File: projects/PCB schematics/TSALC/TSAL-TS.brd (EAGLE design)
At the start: 81.3 x 95.2 mm, 29 parts, among them J1 2P_1-770166-0, J2 2P_1-770166-0, J3 2P_1-770166-0, J4 2P_1-770166-0, X1 5566-2, X2 5566-2

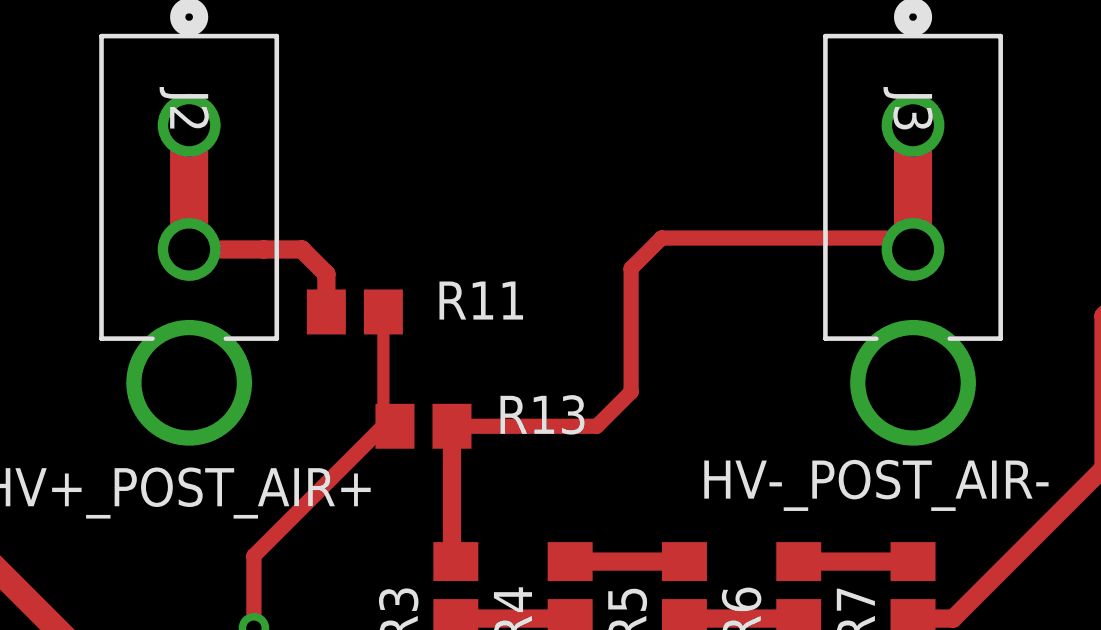
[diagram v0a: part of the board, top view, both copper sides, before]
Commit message: TSAL - Minor fixes.
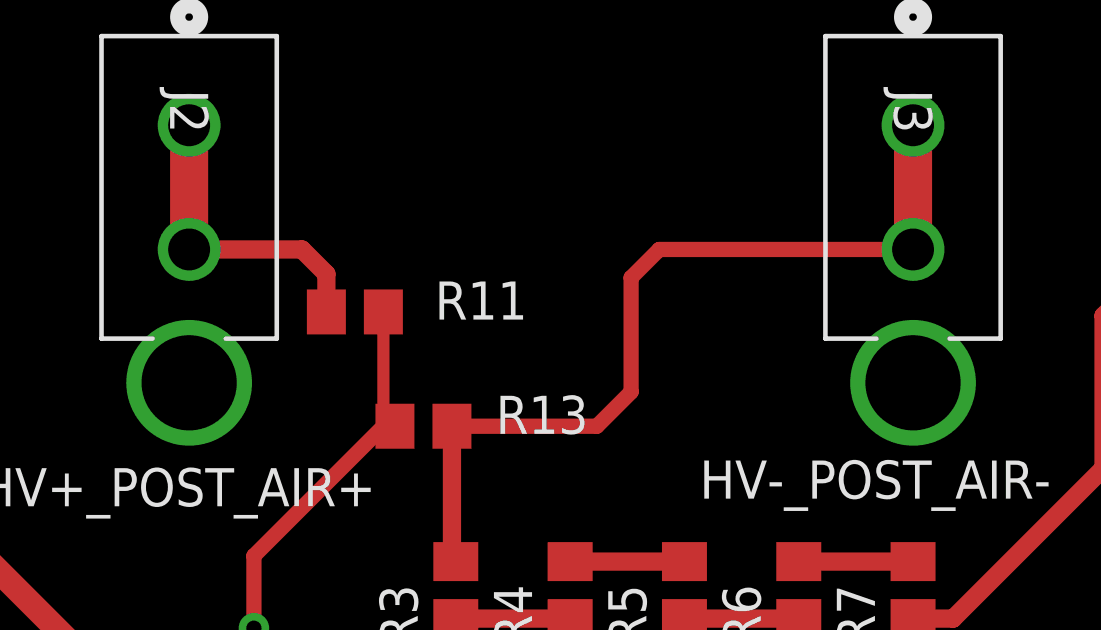
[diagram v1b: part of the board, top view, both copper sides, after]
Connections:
- net HV+_POST_AIR+ renamed MOTORCONTROLLER+
- net HV-_POST_AIR- renamed MOTORCONTROLLER-
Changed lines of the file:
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@@
 <wire x1="33.34" y1="35.24" x2="33.34" y2="33.02" width="0.4064" layer="1"/>
-</signal>
-<signal name="HV+_POST_AIR+">
-<contactref element="R11" pad="2"/>
-<contactref element="J2" pad="1"/>
-<contactref element="J2" pad="2"/>
-<wire x1="27.94" y1="90.17" x2="27.94" y2="86.0298" width="1.27" layer="1"/>
-<wire x1="27.94" y1="86.0298" x2="30.4317" y2="86.0298" width="0.6096" layer="1"/>
-<wire x1="30.4317" y1="86.0298" x2="31.6992" y2="86.0298" width="0.6096" layer="1"/>
-<wire x1="32.5145" y1="85.2145" x2="32.5145" y2="83.947" width="0.6096" layer="1"/>
-<wire x1="31.6992" y1="86.0298" x2="32.5145" y2="85.2145" width="0.6096" layer="1"/>
 </signal>
 <signal name="TSAL_CONTROL_SIGNAL">
@@
 <wire x1="29.1525" y1="53.3975" x2="16.51" y2="66.04" width="0.6096" layer="1"/>
 </signal>
-<signal name="HV-_POST_AIR-">
-<contactref element="J3" pad="1"/>
-<contactref element="J3" pad="2"/>
-<contactref element="R13" pad="1"/>
-<contactref element="R3" pad="1"/>
-<wire x1="52.07" y1="90.17" x2="52.07" y2="86.0298" width="1.27" layer="1"/>
-<wire x1="52.07" y1="86.0298" x2="51.689" y2="86.4108" width="0.508" layer="1"/>
-<wire x1="51.689" y1="86.4108" x2="43.688" y2="86.4108" width="0.508" layer="1"/>
-<wire x1="41.529" y1="80.137" x2="42.672" y2="81.28" width="0.508" layer="1"/>
-<wire x1="42.672" y1="85.3948" x2="43.688" y2="86.4108" width="0.508" layer="1"/>
-<wire x1="36.7005" y1="80.137" x2="41.529" y2="80.137" width="0.508" layer="1"/>
-<wire x1="42.672" y1="81.28" x2="42.672" y2="85.3948" width="0.508" layer="1"/>
-<wire x1="36.83" y1="75.626" x2="36.7005" y2="75.7555" width="0.8128" layer="1"/>
-<wire x1="36.7005" y1="75.7555" x2="36.7005" y2="80.137" width="0.6096" layer="1"/>
-</signal>
 <signal name="N$5">
 <contactref element="R3" pad="2"/>
@@
 <wire x1="46.91" y1="52.15" x2="46.99" y2="52.07" width="0.8128" layer="1"/>
 </signal>
+<signal name="MOTORCONTROLLER+">
+<contactref element="J2" pad="1"/>
+<contactref element="J2" pad="2"/>
+<wire x1="27.94" y1="90.17" x2="27.94" y2="86.0298" width="1.27" layer="1"/>
+<contactref element="R11" pad="2"/>
+<wire x1="32.5145" y1="85.2145" x2="32.5145" y2="83.947" width="0.6096" layer="1"/>
+<wire x1="31.6992" y1="86.0298" x2="32.5145" y2="85.2145" width="0.6096" layer="1"/>
+<wire x1="27.94" y1="86.0298" x2="31.6992" y2="86.0298" width="0.6096" layer="1"/>
+</signal>
+<signal name="MOTORCONTROLLER-">
+<contactref element="J3" pad="1"/>
+<contactref element="J3" pad="2"/>
+<contactref element="R13" pad="1"/>
+<contactref element="R3" pad="1"/>
+<wire x1="41.529" y1="80.137" x2="42.672" y2="81.28" width="0.508" layer="1"/>
+<wire x1="36.7005" y1="80.137" x2="41.529" y2="80.137" width="0.508" layer="1"/>
+<wire x1="42.672" y1="81.28" x2="42.672" y2="85.09" width="0.508" layer="1"/>
+<wire x1="36.83" y1="75.626" x2="36.7005" y2="75.7555" width="0.8128" layer="1"/>
+<wire x1="36.7005" y1="75.7555" x2="36.7005" y2="80.137" width="0.6096" layer="1"/>
+<wire x1="52.07" y1="90.17" x2="52.07" y2="86.0298" width="1.27" layer="1"/>
+<wire x1="42.672" y1="85.09" x2="43.6118" y2="86.0298" width="0.508" layer="1"/>
+<wire x1="43.6118" y1="86.0298" x2="52.07" y2="86.0298" width="0.508" layer="1"/>
+</signal>
 </signals>
